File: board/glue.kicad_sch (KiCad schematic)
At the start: 25 parts, among them J1 Conn_01x05_Pin, J8 SD_Card_Receptacle, U12 GLUE, U13 SN74LVC245APW, U14 LD1117V33

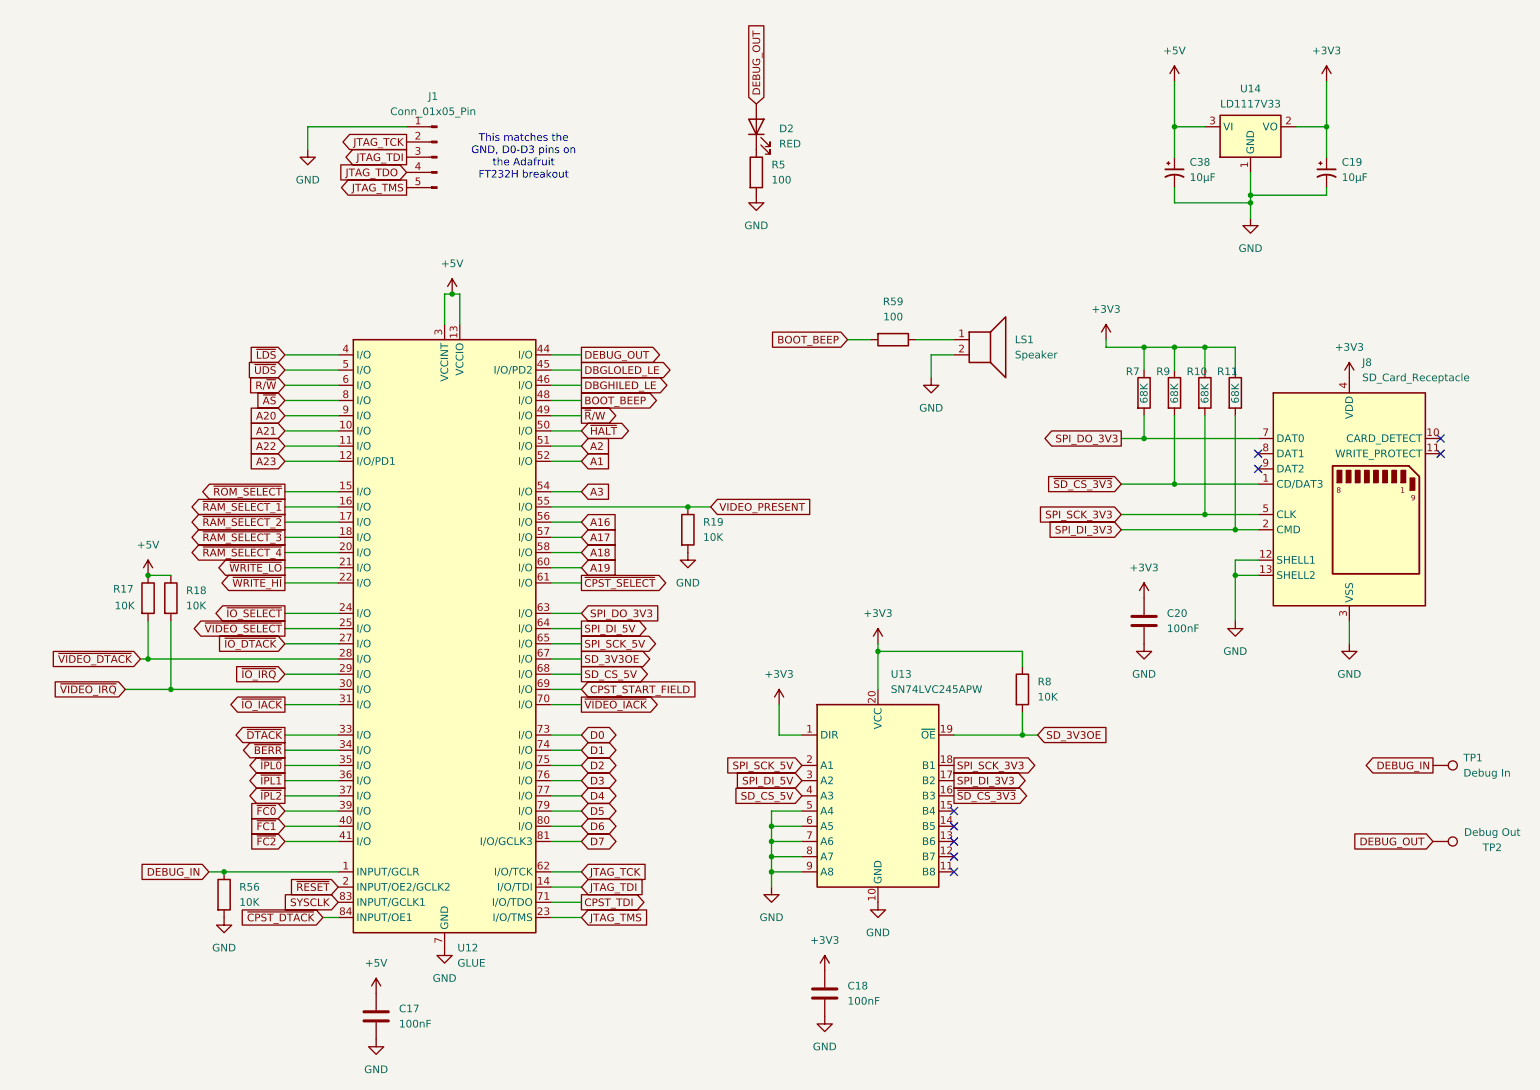
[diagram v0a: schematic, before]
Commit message: checkpoint
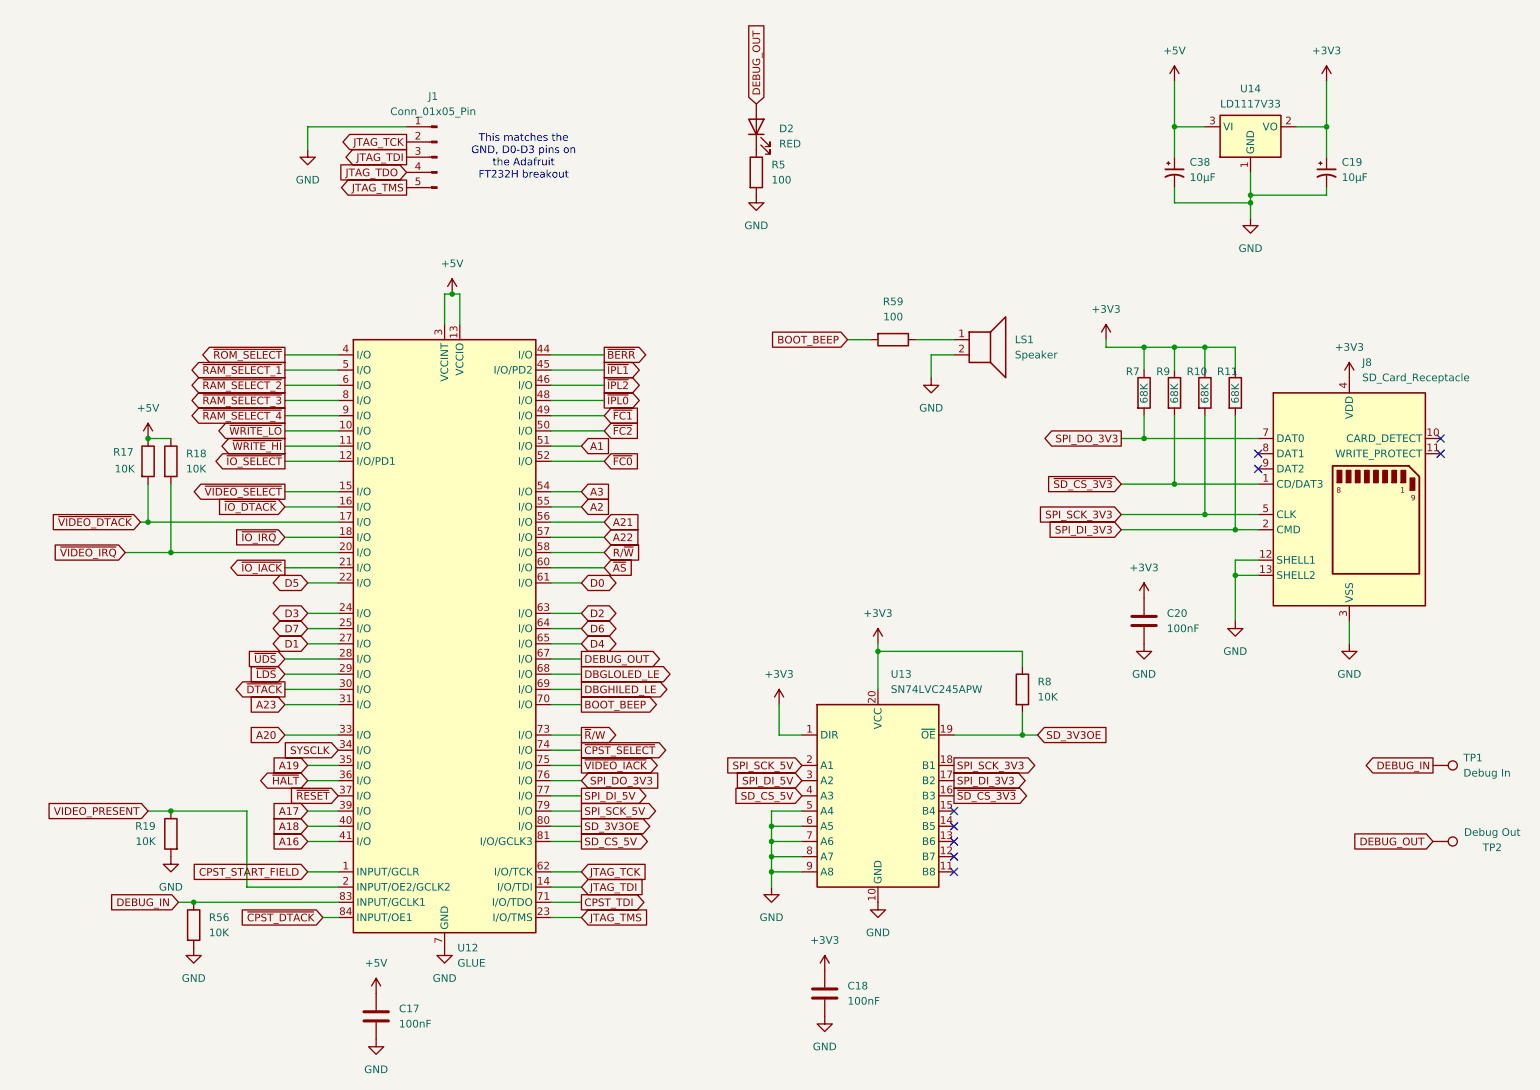
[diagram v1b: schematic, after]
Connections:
- net A1: now also U12.51 (I/O); no longer U12.52 (I/O)
- net A16: now also U12.41 (I/O); no longer U12.56 (I/O)
- net A17: now also U12.39 (I/O); no longer U12.57 (I/O)
- net A18: now also U12.40 (I/O); no longer U12.58 (I/O)
- net A19: now also U12.35 (I/O); no longer U12.60 (I/O)
- net A2: now also U12.55 (I/O); no longer U12.51 (I/O)
- net A20: now also U12.33 (I/O); no longer U12.9 (I/O)
- net A21: now also U12.56 (I/O); no longer U12.10 (I/O)
- net A22: now also U12.57 (I/O); no longer U12.11 (I/O)
- net A23: now also U12.31 (I/O); no longer U12.12 (I/O/PD1)
- net BOOT_BEEP: now also U12.70 (I/O); no longer U12.48 (I/O)
- net CPST_START_FIELD: now also U12.1 (INPUT/GCLR); no longer U12.69 (I/O)
- net D0: now also U12.61 (I/O); no longer U12.73 (I/O)
- net D1: now also U12.27 (I/O); no longer U12.74 (I/O)
- net D2: now also U12.63 (I/O); no longer U12.75 (I/O)
- net D3: now also U12.24 (I/O); no longer U12.76 (I/O)
- net D4: now also U12.65 (I/O); no longer U12.77 (I/O)
- net D5: now also U12.22 (I/O); no longer U12.79 (I/O)
- net D6: now also U12.64 (I/O); no longer U12.80 (I/O)
- net D7: now also U12.25 (I/O); no longer U12.81 (I/O/GCLK3)
- net DBGHILED_LE: now also U12.69 (I/O); no longer U12.46 (I/O)
- net DBGLOLED_LE: now also U12.68 (I/O); no longer U12.45 (I/O/PD2)
- net DEBUG_IN: now also U12.83 (INPUT/GCLK1); no longer U12.1 (INPUT/GCLR)
- net DEBUG_OUT: now also U12.67 (I/O); no longer U12.44 (I/O)
- net R/~{W}: now also U12.58 (I/O); no longer U12.6 (I/O)
- net SD_3V3OE: now also U12.80 (I/O); no longer U12.67 (I/O)
- net SD_CS_5V: now also U12.81 (I/O/GCLK3); no longer U12.68 (I/O)
- net SPI_DI_5V: now also U12.77 (I/O); no longer U12.64 (I/O)
- net SPI_DO_3V3: now also U12.76 (I/O); no longer U12.63 (I/O)
- net SPI_SCK_5V: now also U12.79 (I/O); no longer U12.65 (I/O)
- net SYSCLK: now also U12.34 (I/O); no longer U12.83 (INPUT/GCLK1)
- net VIDEO_PRESENT: now also U12.2 (INPUT/OE2/GCLK2); no longer U12.55 (I/O)
- net ~{AS}: now also U12.60 (I/O); no longer U12.8 (I/O)
- net ~{BERR}: now also U12.44 (I/O); no longer U12.34 (I/O)
- net ~{CPST_SELECT}: now also U12.74 (I/O); no longer U12.61 (I/O)
- net ~{DTACK}: now also U12.30 (I/O); no longer U12.33 (I/O)
- net ~{FC0}: now also U12.52 (I/O); no longer U12.39 (I/O)
- net ~{FC1}: now also U12.49 (I/O); no longer U12.40 (I/O)
- net ~{FC2}: now also U12.50 (I/O); no longer U12.41 (I/O)
- net ~{HALT}: now also U12.36 (I/O); no longer U12.50 (I/O)
- net ~{IO_DTACK}: now also U12.16 (I/O); no longer U12.27 (I/O)
- net ~{IO_IACK}: now also U12.21 (I/O); no longer U12.31 (I/O)
- net ~{IO_IRQ}: now also U12.18 (I/O); no longer U12.29 (I/O)
- net ~{IO_SELECT}: now also U12.12 (I/O/PD1); no longer U12.24 (I/O)
- net ~{IPL0}: now also U12.48 (I/O); no longer U12.35 (I/O)
- net ~{IPL1}: now also U12.45 (I/O/PD2); no longer U12.36 (I/O)
- net ~{IPL2}: now also U12.46 (I/O); no longer U12.37 (I/O)
- net ~{LDS}: now also U12.29 (I/O); no longer U12.4 (I/O)
- net ~{RAM_SELECT_1}: now also U12.5 (I/O); no longer U12.16 (I/O)
- net ~{RAM_SELECT_2}: now also U12.6 (I/O); no longer U12.17 (I/O)
- net ~{RAM_SELECT_3}: now also U12.8 (I/O); no longer U12.18 (I/O)
- net ~{RAM_SELECT_4}: now also U12.9 (I/O); no longer U12.20 (I/O)
- net ~{RESET}: now also U12.37 (I/O); no longer U12.2 (INPUT/OE2/GCLK2)
- net ~{ROM_SELECT}: now also U12.4 (I/O); no longer U12.15 (I/O)
- net ~{R}/W: now also U12.73 (I/O); no longer U12.49 (I/O)
- net ~{UDS}: now also U12.28 (I/O); no longer U12.5 (I/O)
- net ~{VIDEO_DTACK}: now also U12.17 (I/O); no longer U12.28 (I/O)
- net ~{VIDEO_IACK}: now also U12.75 (I/O); no longer U12.70 (I/O)
- net ~{VIDEO_IRQ}: now also U12.20 (I/O); no longer U12.30 (I/O)
- net ~{VIDEO_SELECT}: now also U12.15 (I/O); no longer U12.25 (I/O)
- net ~{WRITE_HI}: now also U12.11 (I/O); no longer U12.22 (I/O)
- net ~{WRITE_LO}: now also U12.10 (I/O); no longer U12.21 (I/O)
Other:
- moved on the sheet: R17, R18, R19, R56

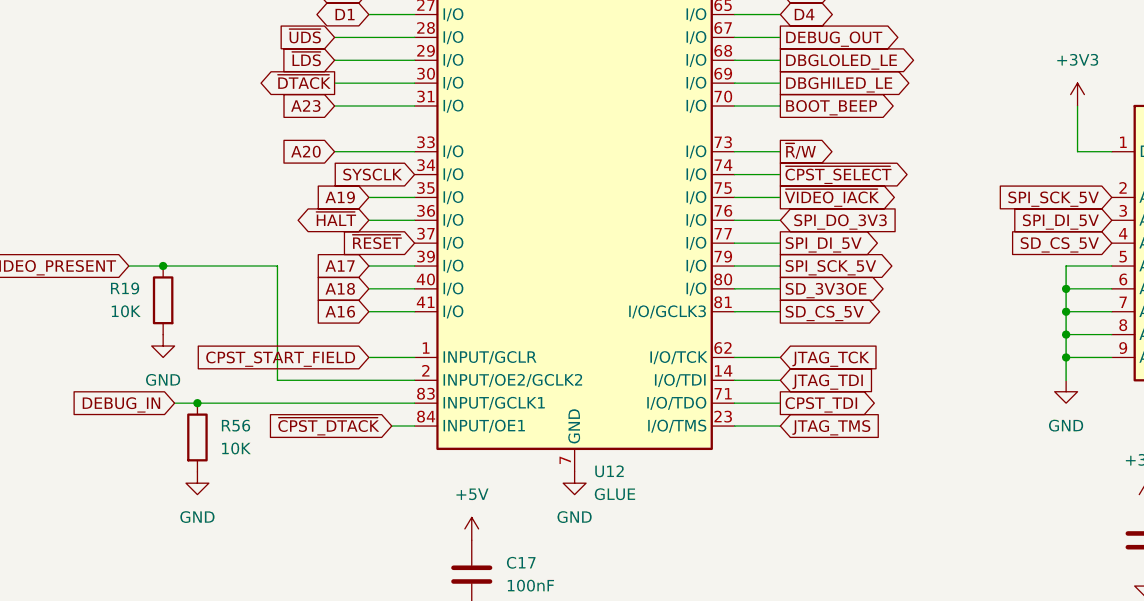
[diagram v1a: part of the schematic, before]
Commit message: checkpoint before deleting composite video
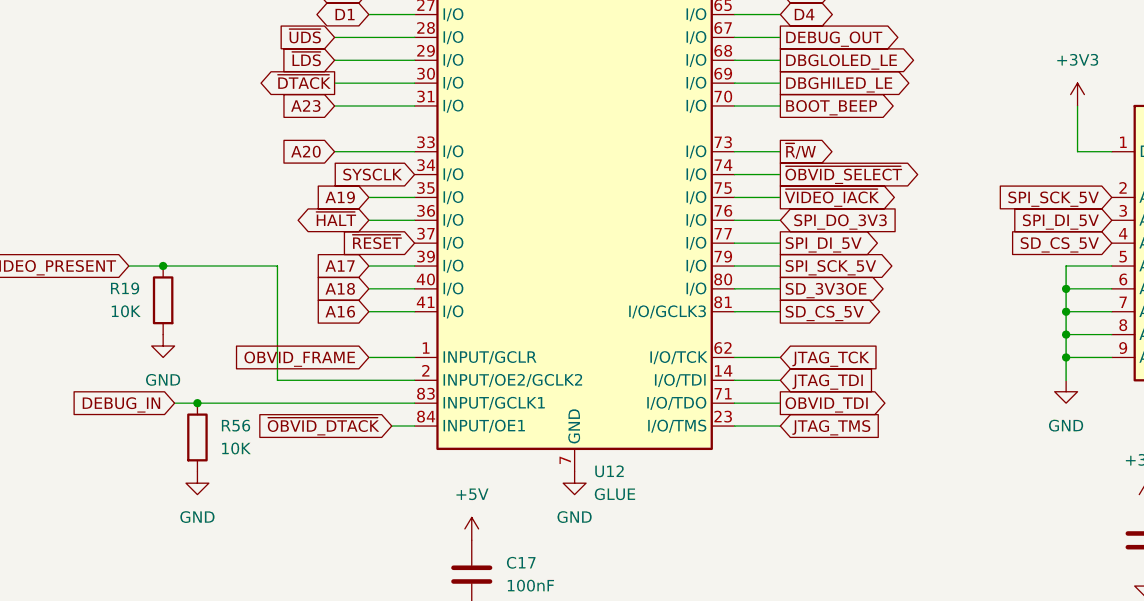
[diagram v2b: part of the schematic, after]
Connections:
- net CPST_START_FIELD renamed OBVID_FRAME
- net CPST_TDI renamed OBVID_TDI
- net ~{CPST_DTACK} renamed ~{OBVID_DTACK}
- net ~{CPST_SELECT} renamed ~{OBVID_SELECT}
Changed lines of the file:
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@@
 		)
 	)
-	(global_label "~{CPST_DTACK}"
+	(global_label "~{OBVID_DTACK}"
 		(shape input)
 		(at 59.69 168.91 180)
@@
 		)
 	)
-	(global_label "CPST_TDI"
+	(global_label "OBVID_TDI"
 		(shape output)
 		(at 102.87 166.37 0)
@@
 		)
 	)
-	(global_label "~{CPST_SELECT}"
+	(global_label "~{OBVID_SELECT}"
 		(shape output)
 		(at 102.87 140.97 0)
@@
 		)
 	)
-	(global_label "CPST_START_FIELD"
+	(global_label "OBVID_FRAME"
 		(shape input)
 		(at 57.15 161.29 180)
